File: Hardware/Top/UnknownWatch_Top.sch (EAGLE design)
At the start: 62 parts, among them SW2 SWITCH.MOM, SW6 SWITCH.MOM, U2 FT231XS, U4 PCF8523, U6 NRF52832_MODULE_MDBT42

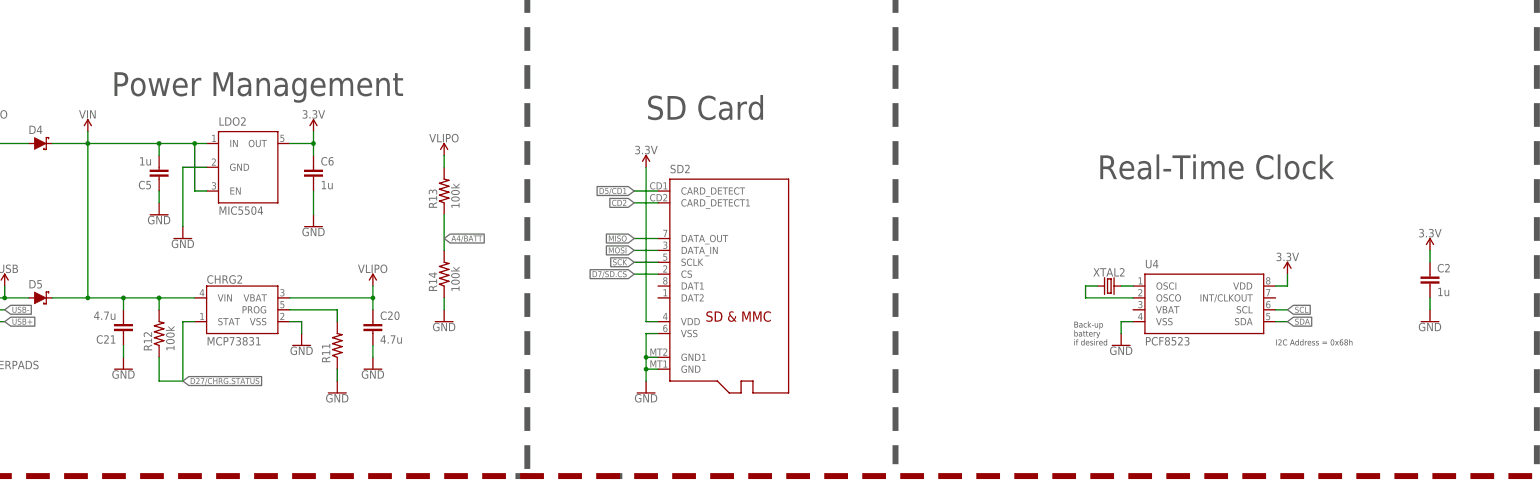
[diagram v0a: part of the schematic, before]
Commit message: Completed take 5 and did part of take 6.
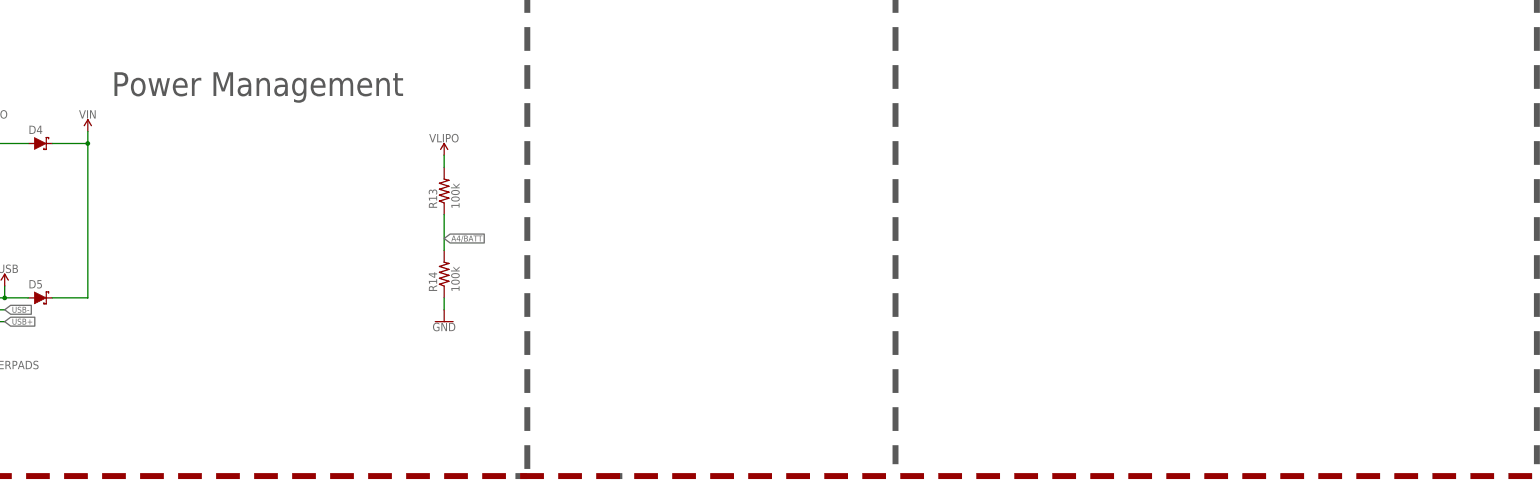
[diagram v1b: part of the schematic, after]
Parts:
- removed C2, C5, C6: 1u, LinnesLab-Passives:CAPACITOR0603
- removed C20, C21: 4.7u, LinnesLab-Passives:CAPACITOR0603
- removed CHRG2: MCP73831, LinnesLab-Power:MCP73831
- removed LDO2: MIC5504, LinnesLab-Power:MIC5504
- removed R11: (no value), LinnesLab-Passives:RESISTOR0603
- removed R12: 100k, LinnesLab-Passives:RESISTOR0603
- removed SD2: (no value), LinnesLab-Connectors:MICROSD
- removed U4: PCF8523, LinnesLab-Clocks:PCF8523
- removed XTAL2: 32.7680kHz, LinnesLab-Clocks:CRYSTALECS-.327-12.5-12-C-TR
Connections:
- removed net CD2: SD2.CARD_DETECT1
- removed net N$17: CHRG2.PROG, R11.2
- removed net N$6: U4.OSCO, XTAL2.1
- removed net N$9: U4.OSCI, XTAL2.2
- net 3.3V: no longer C2.1, C6.1, LDO2.OUT, SD2.VDD, U4.VDD
- net D27/CHRG.STATUS: no longer CHRG2.STAT, R12.1
- net D5/CD1: no longer SD2.CARD_DETECT
- net D7/SD.CS: no longer SD2.CS
- net GND: no longer C2.2, C20.2, C21.1, C5.1, C6.2, CHRG2.VSS, LDO2.GND, R11.1, SD2.GND, SD2.GND1, SD2.VSS, U4.VSS
- net MISO: no longer SD2.DATA_OUT
- net MOSI: no longer SD2.DATA_IN
- net SCK: no longer SD2.SCLK
- net SCL: no longer U4.SCL
- net SDA: no longer U4.SDA
- net VIN: no longer C21.2, C5.2, CHRG2.VIN, LDO2.EN, LDO2.IN, R12.2
- net VLIPO: no longer C20.1, CHRG2.VBAT
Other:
- note removed: "Back-up battery if desired"
- note removed: "I2C Address = 0x68h"
- note removed: "Real-Time Clock"
- note removed: "SD Card"
